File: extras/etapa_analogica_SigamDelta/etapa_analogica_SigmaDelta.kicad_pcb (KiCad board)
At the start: 2 copper layers, 63.5 x 78.8 mm, 18 parts, among them P1 CONN_01X01, P2 CONN_01X01, P3 CONN_01X01, P4 CONN_01X01, P5 CONN_01X02

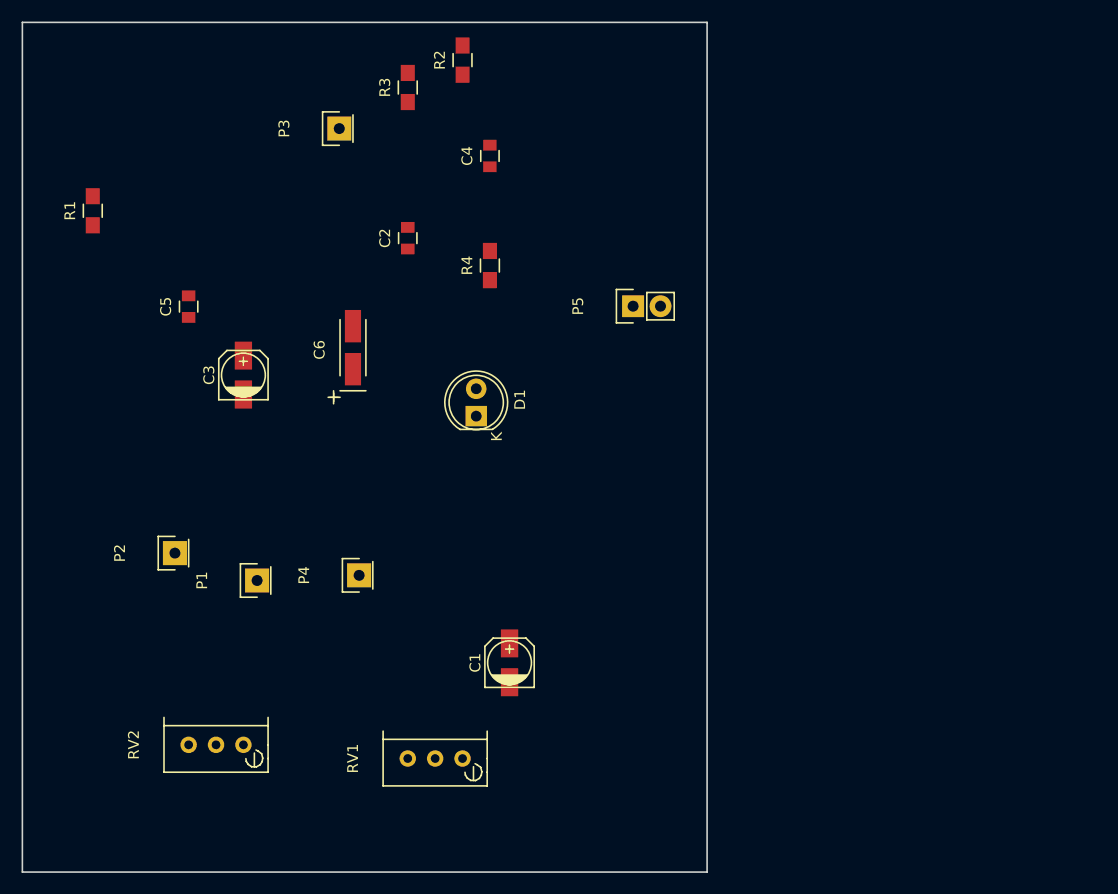
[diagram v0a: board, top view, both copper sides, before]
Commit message: Starting the layout
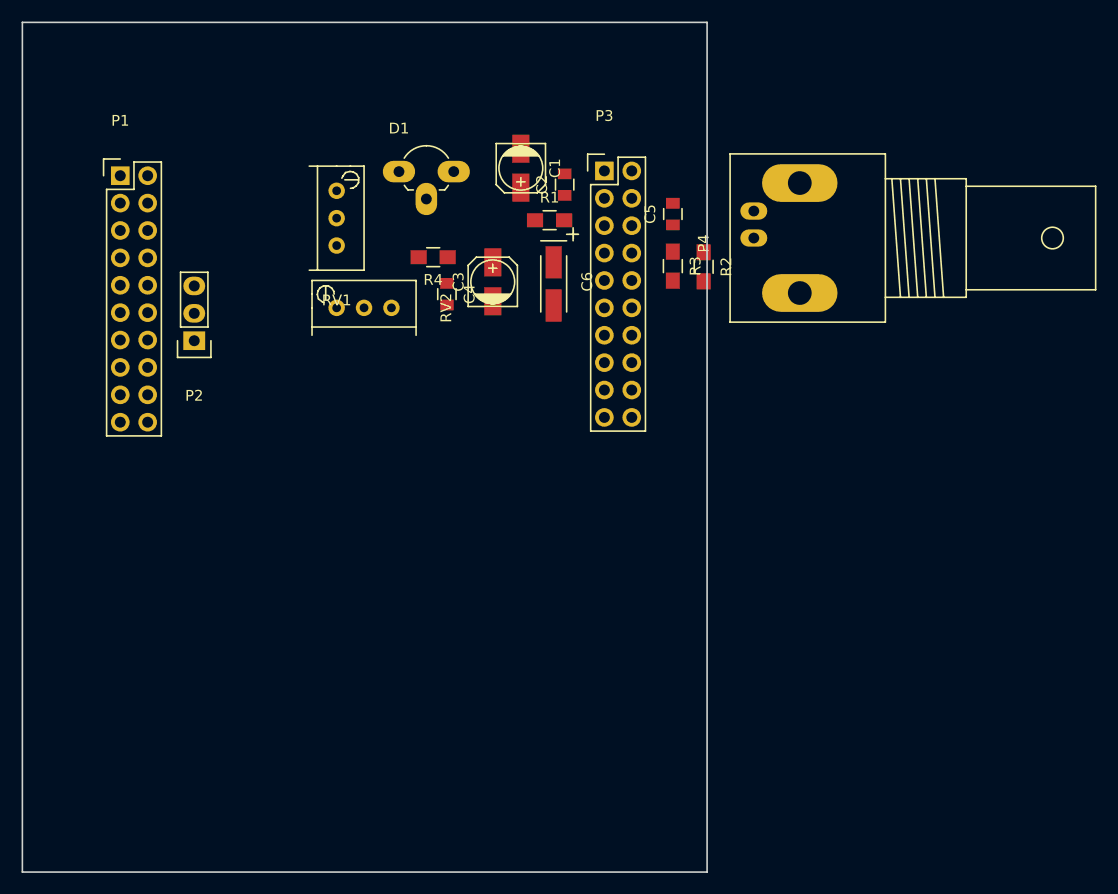
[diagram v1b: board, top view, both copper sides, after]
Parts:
- removed P5: CONN_01X02, Pin_Headers:Pin_Header_Straight_1x02
- D1: footprint LEDs:LED-5MM -> Housings_TO-92:TO-92_Rugged_Reverse
- P1, P3: value CONN_01X01 -> CONN_02X10; footprint Pin_Headers:Pin_Header_Straight_1x01 -> Pin_Headers:Pin_Header_Straight_2x10
- P2: value CONN_01X01 -> CONN_01X03; footprint Pin_Headers:Pin_Header_Straight_1x01 -> Pin_Headers:Pin_Header_Straight_1x03
- P4: value CONN_01X01 -> BNC; footprint Pin_Headers:Pin_Header_Straight_1x01 -> Sockets_BNC:BNC_Socket_TYCO-AMP_LargePads
- RV2: value 1k -> 10k
- moved RV1 53.9 mm to (115.5, 71.4), turned to 180 degrees
- moved P4 52.1 mm to (159.2, 75.8), turned to 270 degrees
- moved C1 45.9 mm to (132.6, 69.3), turned to 270 degrees
- moved C5 45.7 mm to (146.7, 73.6)
- moved R1 42.4 mm to (135.3, 74.2), turned to 0 degrees
- moved RV2 41.4 mm to (115.5, 82.3), turned to 270 degrees
- moved P1 39.6 mm to (95.4, 70.0), turned to 0 degrees
- moved R3 29.6 mm to (146.7, 78.4), turned to 270 degrees
- moved R2 29.5 mm to (149.5, 78.5), turned to 270 degrees
- moved P3 24.9 mm to (140.3, 69.6), turned to 0 degrees
- moved C3 24.7 mm to (130.0, 79.9)
- moved D1 23.8 mm to (121.3, 69.7), turned to 0 degrees
- moved P2 19.8 mm to (102.3, 85.3), turned to 180 degrees
- moved C6 19.5 mm to (135.6, 80.1), turned to 270 degrees
- moved C2 15.4 mm to (136.7, 70.9)
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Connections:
- C1 pad 1: Vcc -> /3,3v
- C2 pad 1: Vcc -> /3,3v
- C3 pad 1: Vref -> /N40
- C4 pad 1: Vref -> /N40
- C5 pad 1: Vin -> /P41
- C6 pad 1: Vref -> /N40
- D1 pad 1: Net-(D1-Pad1) -> GND
- D1 pad 2: GND -> Net-(D1-Pad2)
- P1 pad 1: Vsignal -> Net-(P1-Pad1)
- P2 pad 1: GND -> /Tx
- P3 pad 1: Vfb -> Net-(P3-Pad1)
- P4 pad 1: Vcc -> Net-(P4-Pad1)
- R1 pad 1: Net-(D1-Pad1) -> Net-(D1-Pad2)
- R1 pad 2: Vcc -> /3,3v
- R2 pad 1: Vin -> /P41
- R2 pad 2: Vsignal -> Net-(P4-Pad1)
- R3 pad 1: Vin -> /P41
- R3 pad 2: Vfb -> /P35
- R4 pad 1: Vref -> /N40
- RV1 pad 1: Net-(D1-Pad1) -> Net-(D1-Pad2)
- RV1 pad 2: Net-(R4-Pad2) -> Net-(RV1-Pad2)
- RV1 pad 3: Net-(RV1-Pad3) -> Net-(RV1-Pad2)
- RV2 pad 1: Net-(RV1-Pad3) -> Net-(RV1-Pad2)
- RV2 pad 2: GND -> Net-(R4-Pad2)
